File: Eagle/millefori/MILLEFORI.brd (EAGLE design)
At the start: 72.7 x 47 mm, 18 parts

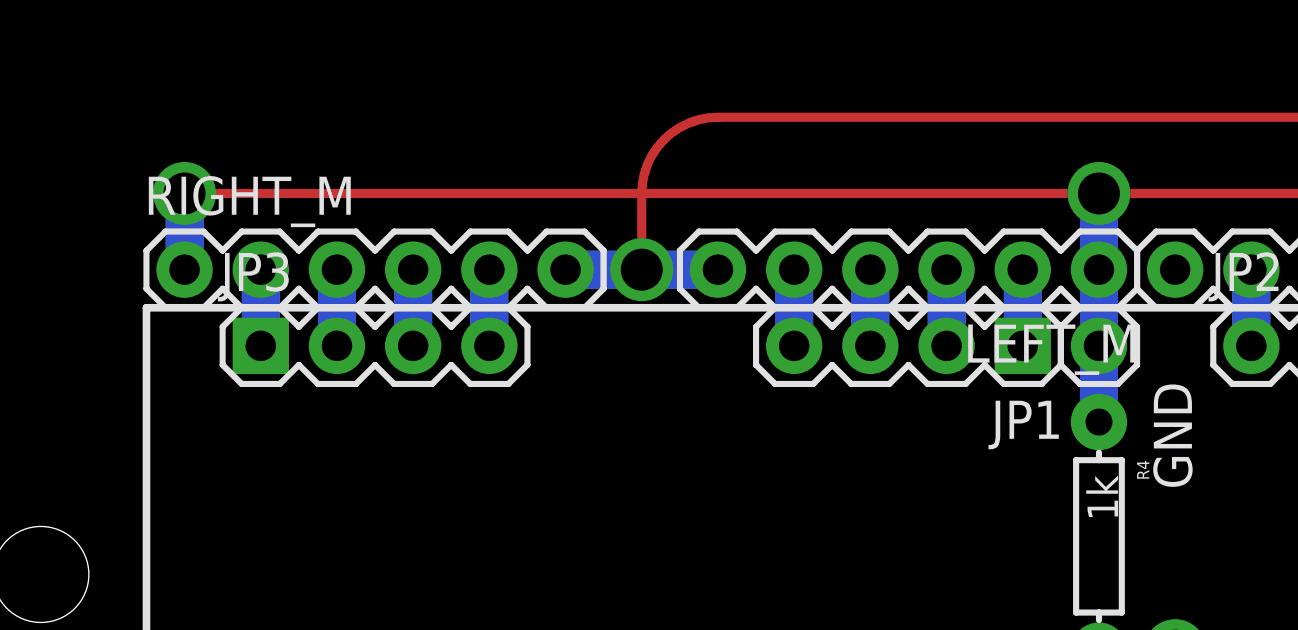
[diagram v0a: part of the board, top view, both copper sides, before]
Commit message: SCHEMA ELETTRICO
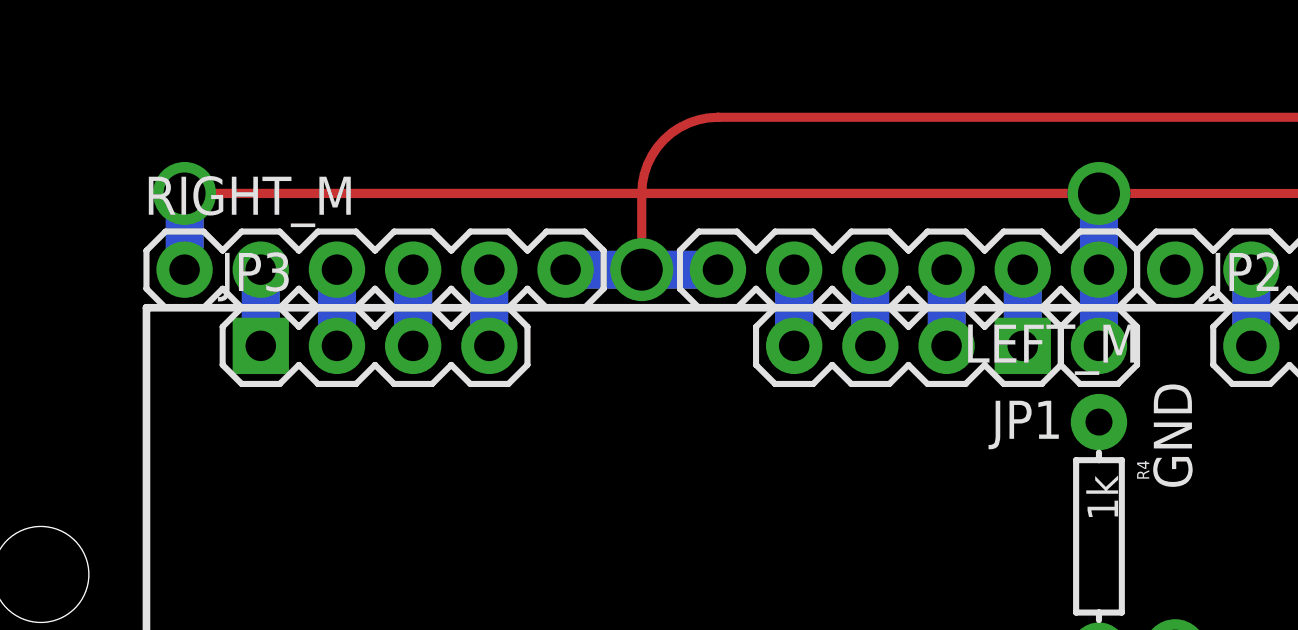
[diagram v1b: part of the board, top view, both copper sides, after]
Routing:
- net GND: track 161.0 -> 188.9 mm
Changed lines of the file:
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@@
 <layer number="19" name="Unrouted" color="6" fill="1" visible="no" active="yes"/>
 <layer number="20" name="Dimension" color="15" fill="1" visible="yes" active="yes"/>
-<layer number="21" name="tPlace" color="7" fill="1" visible="no" active="yes"/>
+<layer number="21" name="tPlace" color="7" fill="1" visible="yes" active="yes"/>
 <layer number="22" name="bPlace" color="7" fill="1" visible="no" active="yes"/>
 <layer number="23" name="tOrigins" color="15" fill="1" visible="no" active="yes"/>
@@
 <layer number="44" name="Drills" color="7" fill="1" visible="yes" active="yes"/>
 <layer number="45" name="Holes" color="7" fill="1" visible="no" active="yes"/>
-<layer number="46" name="Milling" color="3" fill="1" visible="yes" active="yes"/>
+<layer number="46" name="Milling" color="3" fill="1" visible="no" active="yes"/>
 <layer number="47" name="Measures" color="7" fill="1" visible="no" active="yes"/>
 <layer number="48" name="Document" color="7" fill="1" visible="yes" active="yes"/>
-<layer number="49" name="Reference" color="7" fill="1" visible="yes" active="yes"/>
+<layer number="49" name="Reference" color="7" fill="1" visible="no" active="yes"/>
 <layer number="50" name="dxf" color="7" fill="1" visible="no" active="no"/>
-<layer number="51" name="tDocu" color="7" fill="1" visible="yes" active="yes"/>
-<layer number="52" name="bDocu" color="7" fill="1" visible="yes" active="yes"/>
+<layer number="51" name="tDocu" color="7" fill="1" visible="no" active="yes"/>
+<layer number="52" name="bDocu" color="7" fill="1" visible="no" active="yes"/>
 <layer number="53" name="tGND_GNDA" color="7" fill="9" visible="no" active="no"/>
 <layer number="54" name="bGND_GNDA" color="1" fill="9" visible="no" active="no"/>
@@
 <wire x1="20.32" y1="40.64" x2="20.32" y2="5.08" width="0" layer="47"/>
 <wire x1="17.78" y1="5.08" x2="17.78" y2="40.64" width="0" layer="47"/>
-<text x="25.4" y="31.115" size="1.778" layer="27" rot="R270" align="center-left">D12</text>
-<text x="25.4" y="20.32" size="1.778" layer="27" rot="R90" align="center-left">D13</text>
-<text x="60.96" y="31.115" size="1.778" layer="27" rot="R270" align="center-left">TX</text>
-<text x="58.42" y="31.115" size="1.778" layer="27" rot="R270" align="center-left">RX</text>
-<text x="50.8" y="31.115" size="1.778" layer="27" rot="R270" align="center-left">D2</text>
-<text x="48.26" y="31.115" size="1.778" layer="27" rot="R270" align="center-left">D3</text>
-<text x="45.72" y="31.115" size="1.778" layer="27" rot="R270" align="center-left">D4</text>
-<text x="43.18" y="31.115" size="1.778" layer="27" rot="R270" align="center-left">D5</text>
-<text x="33.02" y="31.115" size="1.778" layer="27" rot="R270" align="center-left">D9</text>
-<text x="30.48" y="31.115" size="1.778" layer="27" rot="R270" align="center-left">D10</text>
-<text x="27.94" y="31.115" size="1.778" layer="27" rot="R270" align="center-left">D11</text>
-<text x="69.215" y="11.43" size="1.778" layer="27" rot="R180" align="center-left">GND</text>
+<text x="25.4" y="29.21" size="1.778" layer="27" rot="R270" align="center-left">D12</text>
+<text x="24.13" y="12.7" size="1.778" layer="27" rot="R180" align="center-left">D13</text>
+<text x="60.96" y="29.21" size="1.778" layer="27" rot="R270" align="center-left">TX</text>
+<text x="58.42" y="29.21" size="1.778" layer="27" rot="R270" align="center-left">RX</text>
+<text x="50.8" y="29.21" size="1.778" layer="27" rot="R270" align="center-left">D2</text>
+<text x="48.26" y="29.21" size="1.778" layer="27" rot="R270" align="center-left">D3</text>
+<text x="45.72" y="29.21" size="1.778" layer="27" rot="R270" align="center-left">D4</text>
+<text x="43.18" y="29.21" size="1.778" layer="27" rot="R270" align="center-left">D5</text>
+<text x="33.02" y="29.21" size="1.778" layer="27" rot="R270" align="center-left">D9</text>
+<text x="30.48" y="29.21" size="1.778" layer="27" rot="R270" align="center-left">D10</text>
+<text x="27.94" y="29.21" size="1.778" layer="27" rot="R270" align="center-left">D11</text>
+<text x="69.215" y="8.89" size="1.778" layer="27" rot="R180" align="center-left">GND</text>
 <text x="62.23" y="15.24" size="1.778" layer="27" align="center-left">VIN</text>
-<text x="67.31" y="31.115" size="1.778" layer="27" rot="R270" align="center-left">5V</text>
-<text x="33.02" y="21.59" size="1.778" layer="27" rot="R90" align="center-left">A7</text>
-<text x="51.435" y="17.78" size="1.778" layer="27" rot="R180" align="center-left">A0</text>
-<text x="57.15" y="24.13" size="1.778" layer="27" align="center-left">5V</text>
-<text x="38.735" y="40.64" size="1.778" layer="27" rot="R180" align="center-left">VIN</text>
-<text x="23.495" y="10.16" size="1.778" layer="27" rot="R180" align="center-left">GND</text>
-<text x="23.495" y="13.335" size="1.778" layer="27" rot="R180" align="center-left">5V</text>
+<text x="67.31" y="30.48" size="1.778" layer="27" align="center-left">5V</text>
+<text x="34.29" y="15.24" size="1.778" layer="27" align="center-left">A7</text>
+<text x="52.07" y="15.24" size="1.778" layer="27" rot="R180" align="center-left">A0</text>
+<text x="54.61" y="11.43" size="1.778" layer="27" rot="R180" align="center-left">5V</text>
+<text x="40.64" y="30.48" size="1.778" layer="27" rot="R180" align="center-left">VIN</text>
+<text x="24.13" y="7.62" size="1.778" layer="27" rot="R180" align="center-left">GND</text>
+<text x="24.13" y="10.16" size="1.778" layer="27" rot="R180" align="center-left">5V</text>
+<text x="31.115" y="36.83" size="1.778" layer="27" rot="R180" align="center-left">GND</text>
+<text x="51.435" y="36.83" size="1.778" layer="27" rot="R180" align="center-left">GND</text>
+<text x="61.595" y="36.83" size="1.778" layer="27" rot="R180" align="center-left">GND</text>
+<text x="69.85" y="39.37" size="1.778" layer="27" rot="R180" align="center-left">VIN</text>
 </plain>
 <attributes>
@@
 <contactref element="R4" pad="P$1"/>
 <contactref element="SERVO" pad="3"/>
-<wire x1="53.34" y1="27.94" x2="53.34" y2="30.48" width="1.27" layer="16"/>
+<wire x1="53.34" y1="27.94" x2="53.34" y2="30.48" width="0" layer="19" extent="1-16"/>
 <via x="71.12" y="7.62" extent="1-16" drill="1.4" diameter="1.27" shape="square"/>
 <via x="58.42" y="12.7" extent="1-16" drill="1.4" diameter="1.27" shape="square"/>
@@
 <wire x1="81.785" y1="12.725" x2="82.42" y2="13.36" width="1.27" layer="1" curve="90"/>
 <wire x1="68.58" y1="35.56" x2="63.5" y2="35.56" width="0" layer="19" extent="1-1"/>
+<wire x1="22.86" y1="35.56" x2="53.34" y2="35.56" width="0.3048" layer="1"/>
 </signal>
 <signal name="D13">
